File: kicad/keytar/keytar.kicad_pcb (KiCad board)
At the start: 2 copper layers, 76 x 95 mm, 12 parts, among them J1 , J2 USB_B, J3 Conn_01x02, J4 Conn_01x04, U1 Pico

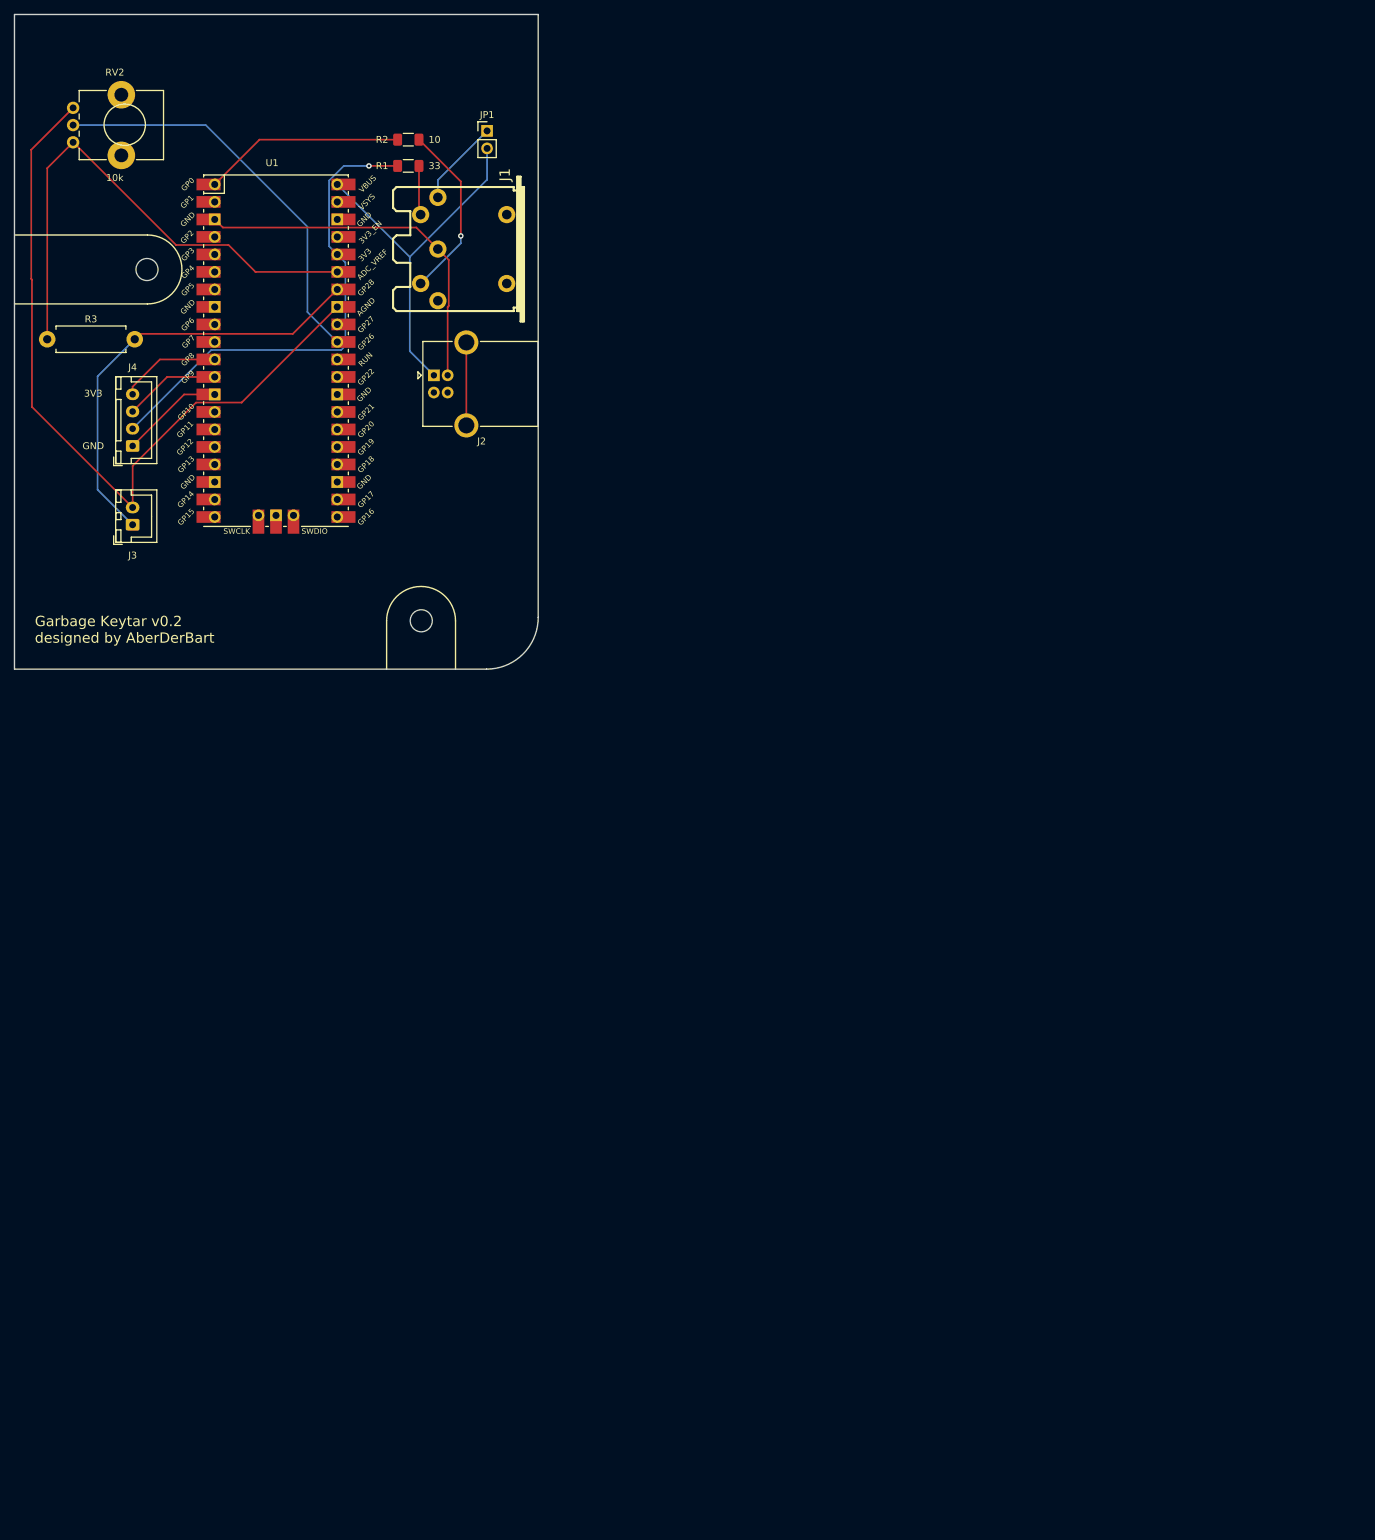
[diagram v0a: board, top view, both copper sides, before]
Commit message: redesign pcb
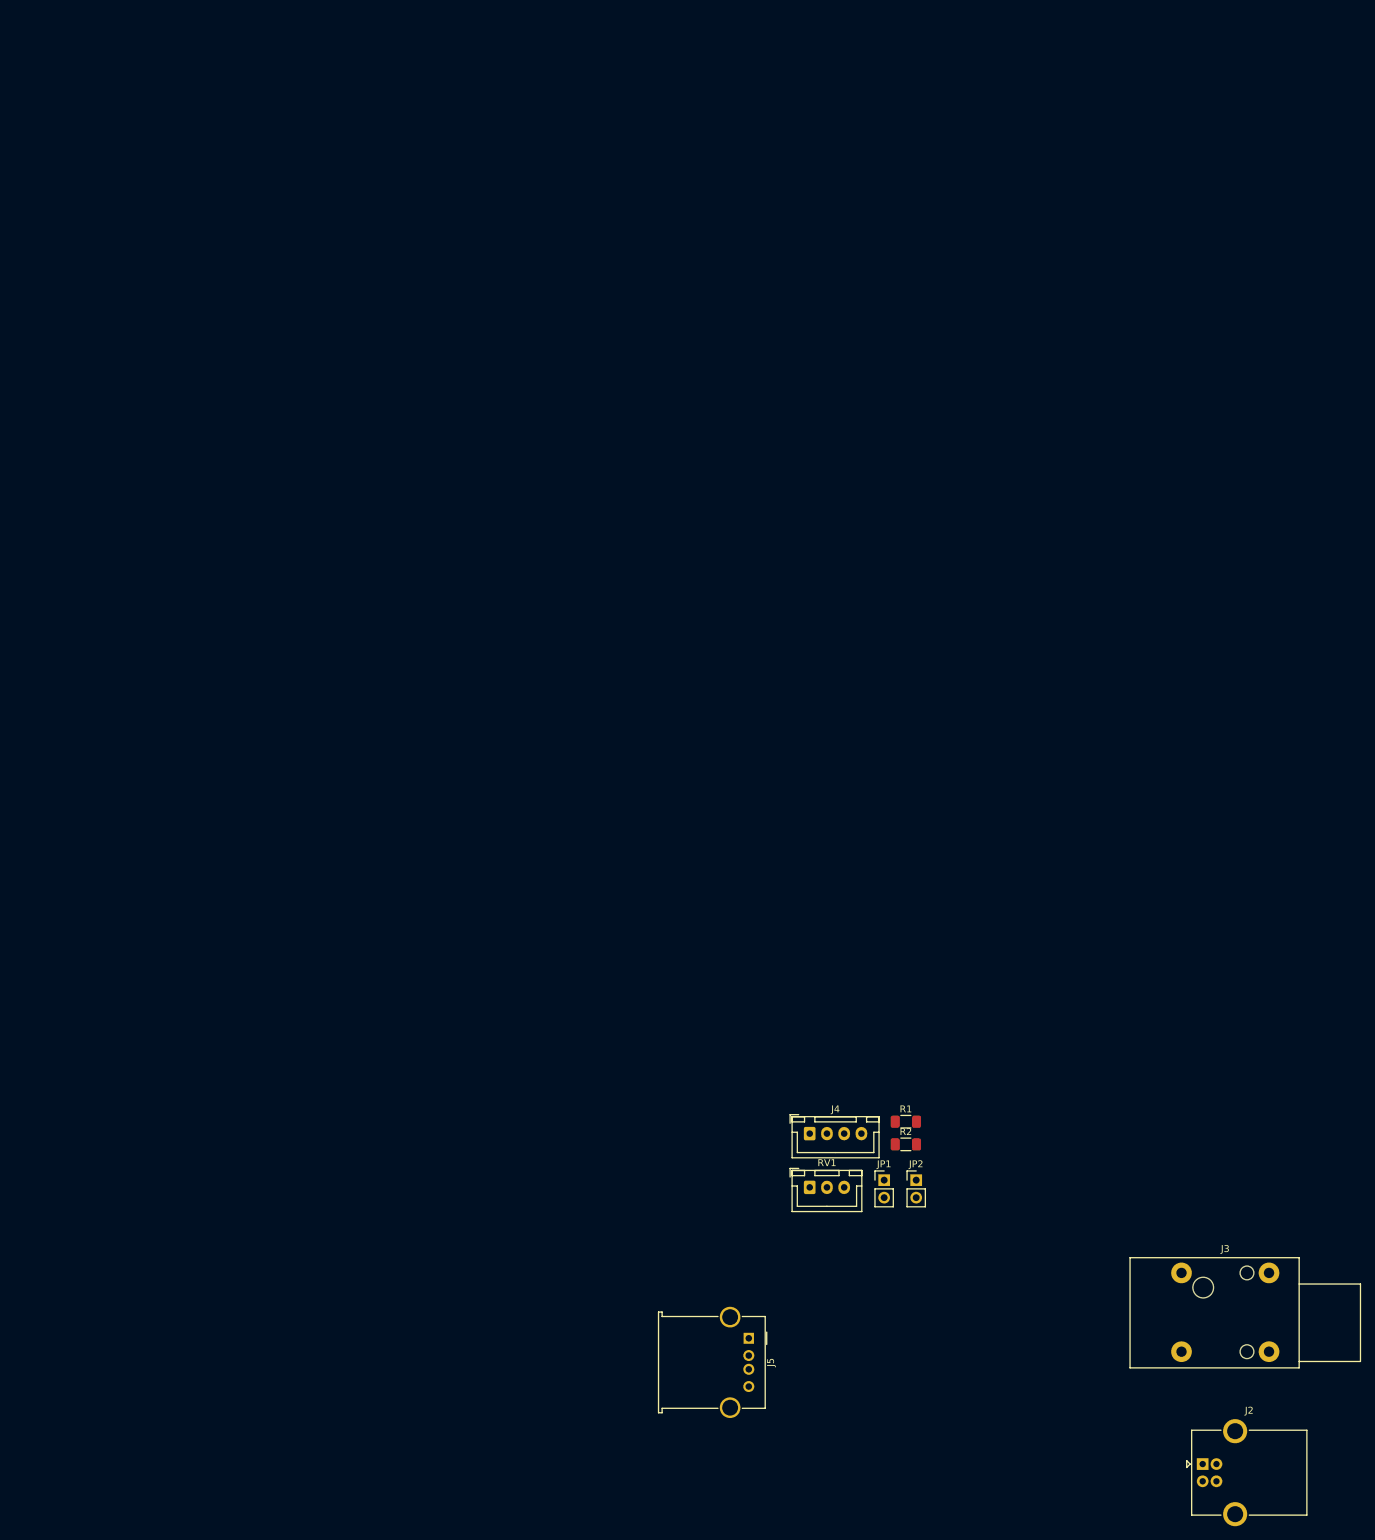
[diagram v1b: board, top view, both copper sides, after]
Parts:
- removed  : MountingHole_3.2mm_M3, MountingHole:MountingHole_3.2mm_M3 (x2)
- removed J1: , Eurocad:MIDI_DIN5
- removed R3: R, Resistor_THT:R_Axial_DIN0411_L9.9mm_D3.6mm_P12.70mm_Horizontal
- removed RV2: 10k, Potentiometer_THT:Potentiometer_Alps_RK09K_Single_Vertical
- removed U1: Pico, MCU_RaspberryPi_and_Boards:RPi_Pico_SMD_TH
- added J5: USB_A, Connector_USB:USB_A_Molex_67643_Horizontal, F.Cu at (106.6, 97.1)
- added JP2: USB Power, Connector_PinHeader_2.54mm:PinHeader_1x02_P2.54mm_Vertical, F.Cu at (130.8, 74.2)
- added RV1: R_POT, Connector_JST:JST_XH_B3B-XH-A_1x03_P2.50mm_Vertical, F.Cu at (115.4, 75.2)
- J3: value Conn_01x02 -> AudioJack2; footprint Connector_JST:JST_XH_B2B-XH-A_1x02_P2.50mm_Vertical -> Connector_Audio:Jack_6.35mm_Neutrik_NRJ4HF_Horizontal
- JP1: value Jumper -> MIDI Power
- moved J2 193.4 mm to (172.4, 115.3)
- moved J3 187.0 mm to (169.3, 87.6), turned to 0 degrees
- moved JP1 162.8 mm to (126.2, 74.2)
- moved R2 162.7 mm to (129.3, 69.0), turned to 0 degrees
- moved R1 156.4 mm to (129.3, 65.7), turned to 0 degrees
- moved J4 140.0 mm to (115.4, 67.4), turned to 0 degrees
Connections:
- net Net-(J4-Pad2) renamed +3V3
- J2 pad 1: Net-(J2-Pad1) -> Net-(J2-VBUS)
- J2 pad 2: Net-(J2-Pad2) -> unconnected-(J2-D--Pad2)
- J2 pad 3: Net-(J2-Pad3) -> unconnected-(J2-D+-Pad3)
- J2 pad 5: Net-(J2-Pad5) -> unconnected-(J2-Shield-Pad5)
- J4 pad 1: Net-(J4-Pad1) -> GND
- JP1 pad 2: Net-(J2-Pad1) -> +5V
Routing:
- net Net-(J3-Pad2): track 111.9 -> 0.00 mm
- net Net-(R3-Pad1): track 76.3 -> 0.00 mm
- net +3V3: track 71.6 -> 0.00 mm, vias 1 -> 0
- net Net-(J3-Pad1): track 64.7 -> 0.00 mm
- net Net-(RV2-Pad2): track 58.6 -> 0.00 mm
- net Net-(J2-Pad1): track 53.9 -> 0.00 mm
- net GND: track 53.2 -> 0.00 mm
- net Net-(U1-GPIO0): track 29.2 -> 0.00 mm
- net Net-(J1-Pad5): track 25.8 -> 0.00 mm, vias 1 -> 0
- net Net-(J4-Pad1): track 15.0 -> 0.00 mm
- net Net-(J4-Pin_4): track 14.7 -> 0.00 mm
- net Net-(J4-Pin_3): track 14.0 -> 0.00 mm
- net Net-(J1-Pad1): track 12.6 -> 0.00 mm
- net Net-(J2-Pad5): track 12.0 -> 0.00 mm
- net Net-(J1-Pad4): track 7.17 -> 0.00 mm
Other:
- board outline removed
- net class Default removed
- board text removed: "3V3"
- board text removed: "GND"
- board text removed: "Garbage Keytar v0.2 designed by AberDerBart"
